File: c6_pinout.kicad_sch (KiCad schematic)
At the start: 19 parts, among them J4 Conn_01x08_Socket, J5 Conn_01x06_Socket, J6 Conn_01x04, J7 Conn_01x10_Socket, J8 Conn_01x06_Socket, U4 ESP32-C6-WROOM-1-N8

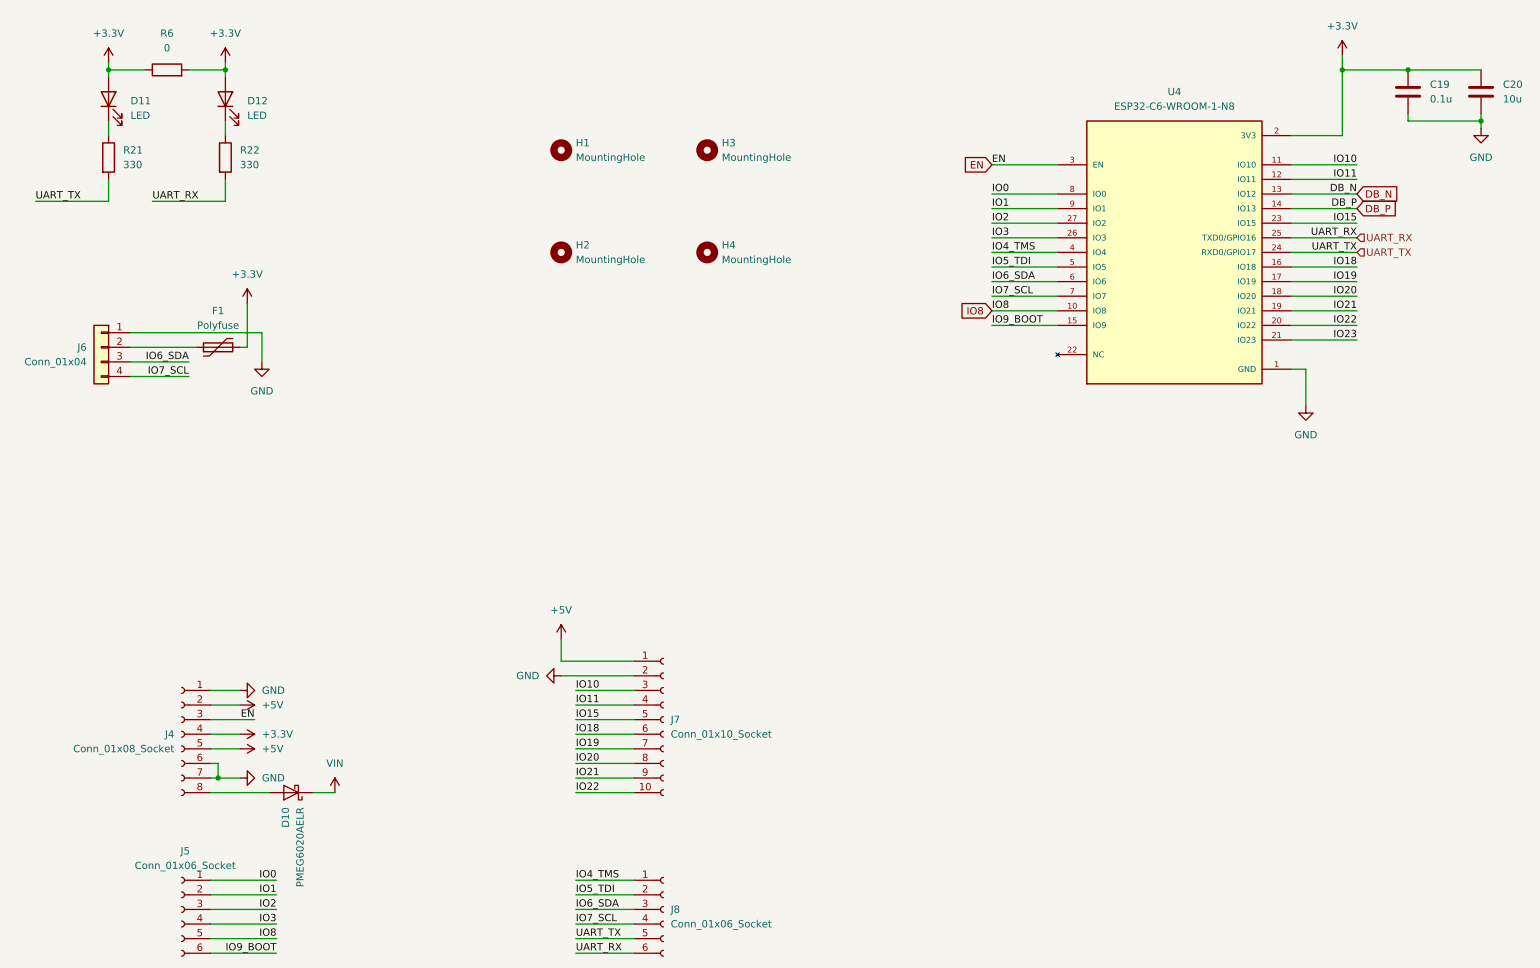
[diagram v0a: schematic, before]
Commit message: Refinement to pcb and schematic layout
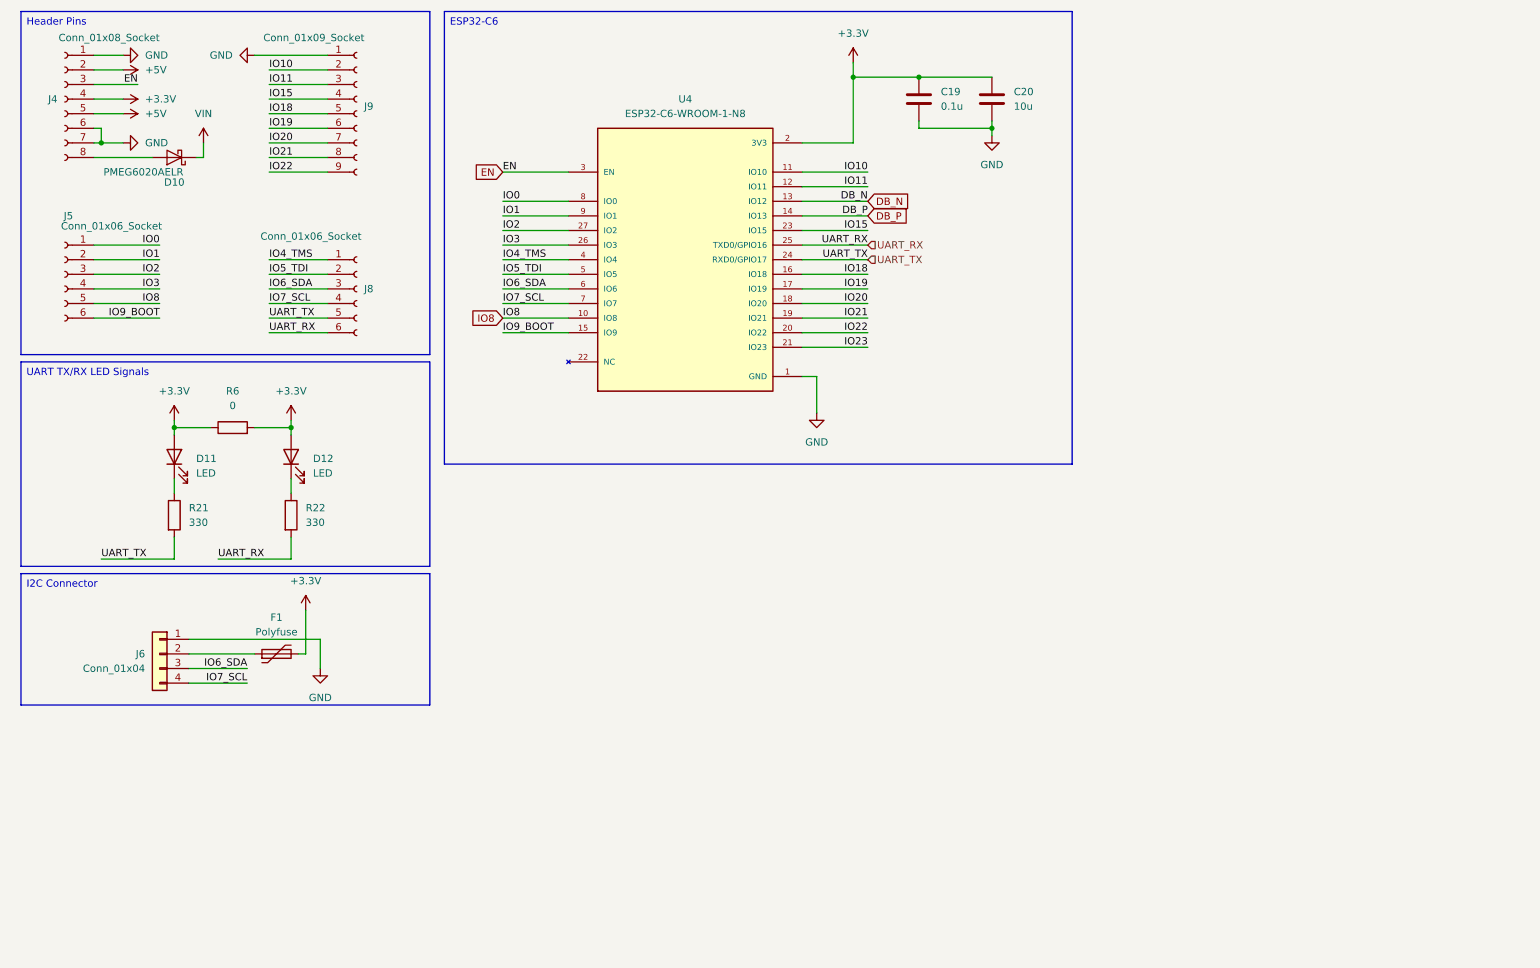
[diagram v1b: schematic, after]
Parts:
- removed H1, H2, H3, H4: MountingHole, MountingHole:MountingHole_2.1mm, symbol Mechanical:MountingHole
- removed J7: Conn_01x10_Socket, Connector_PinSocket_2.00mm:PinSocket_1x10_P2.00mm_Vertical, symbol Connector:Conn_01x10_Socket
- added J9: Conn_01x09_Socket, Connector_PinSocket_2.00mm:PinSocket_1x09_P2.00mm_Vertical, symbol Connector:Conn_01x09_Socket
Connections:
- net GND: now also J9.1 (Pin_1)
- net IO10: now also J9.2 (Pin_2)
- net IO11: now also J9.3 (Pin_3)
- net IO15: now also J9.4 (Pin_4)
- net IO18: now also J9.5 (Pin_5)
- net IO19: now also J9.6 (Pin_6)
- net IO20: now also J9.7 (Pin_7)
- net IO21: now also J9.8 (Pin_8)
- net IO22: now also J9.9 (Pin_9)
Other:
- title: (none) -> ESP32-C6 Dev Board
- moved on the sheet: C19, C20, D10, D11, D12, F1, J4, J5, J6, J8, R21, R22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
